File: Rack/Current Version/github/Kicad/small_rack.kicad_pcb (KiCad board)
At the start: 4 copper layers, 188 parts, among them J1 MOLEX_0015244745, J1001 HOLE_BP, J1002 HOLE_BP, J1003 HOLE_BP, J1004 HOLE_BP, J1005 HOLE_BP, J1006 HOLE_BP, J1007 HOLE_BP, J1008 HOLE_BP, J1009 HOLE_BP, J1010 HOLE_BP, J1011 HOLE_BP, J1012 HOLE_BP, J1013 HOLE_BP, J1014 HOLE_BP, J1015 HOLE_BP, J1016 HOLE_BP, J1017 HOLE_BP, J1018 HOLE_BP, J1019 HOLE_BP, J1020 HOLE_BP, J1021 SLIDER, J1022 SLIDER, J2 USB_CONNEC, K1 CONN_3, P1 CONN_8, U1 USB_CONNEC, U10 SN65LVDM176DGK, U11 TPS2044BDR, U12 CY7C65631-56LTXC, U13 USBLC6-2, U14 USBLC6-2, U15 USBLC6-2, U16 USBLC6-2, U17 USBLC6-2, U18 TPS2044BDR, U19 CY7C65631-56LTXC, U2 TE-8-1393640-3, U20 USBLC6-2, U21 USBLC6-2, U22 USBLC6-2, U23 USBLC6-2, U24 USBLC6-2, U25 CUBIEBOARD, U26 NCP1117, U27 LM73-0, U28 ATMEGA32U4, U29 ACS713, U3 TE-8-1393640-3, U4 R-535.0PA, U5 MAX1685, U6 TE-8-1393640-3, U7 TE-8-1393640-3, U8 TE-8-1393640-3, U9 FOX924B, X1 24MHz, X2 24MHz, X3 16MHz

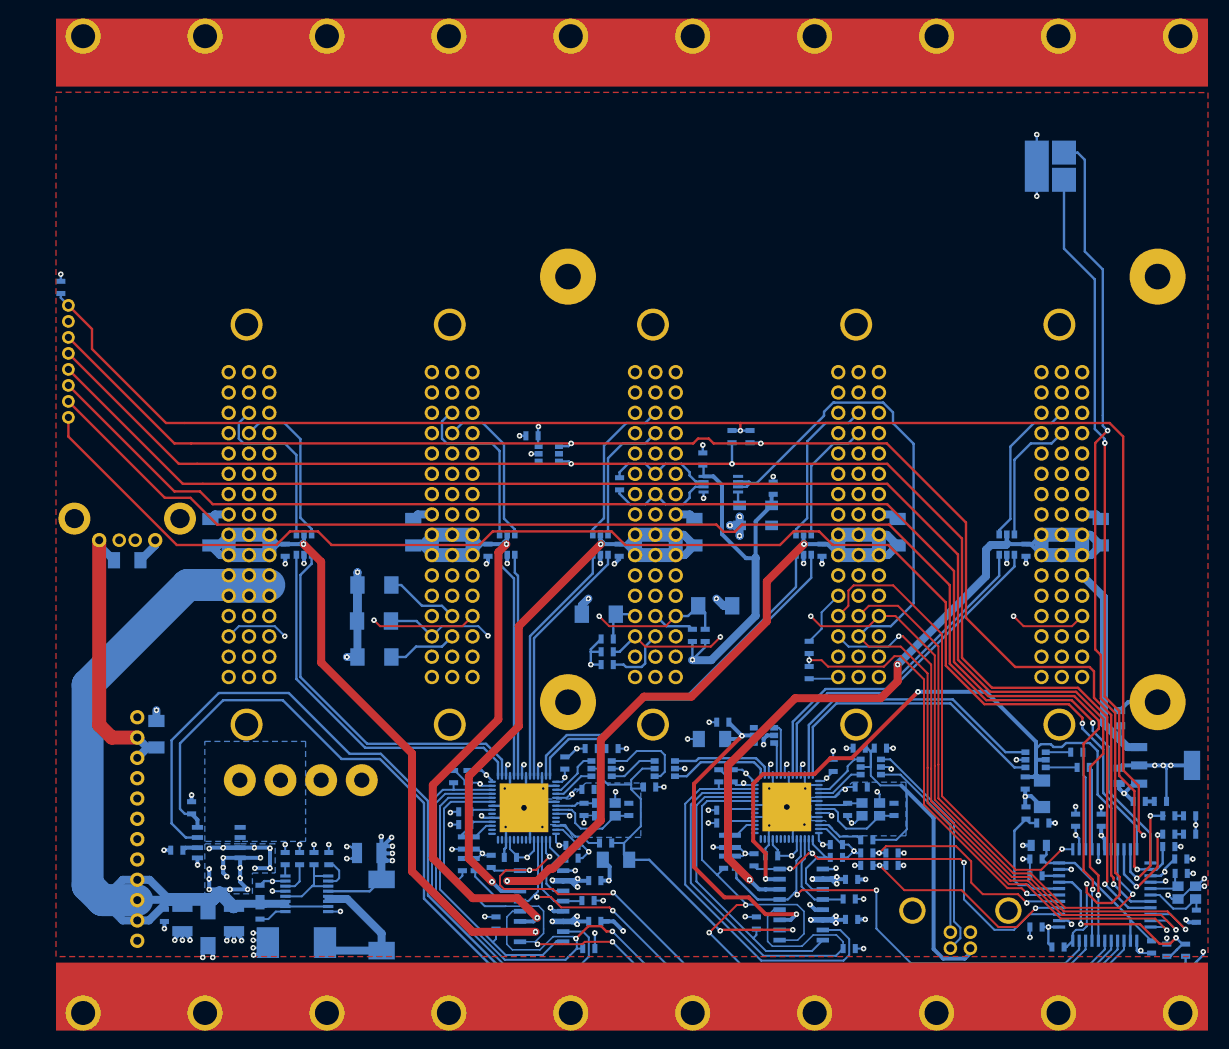
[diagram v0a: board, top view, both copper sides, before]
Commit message: current rack files
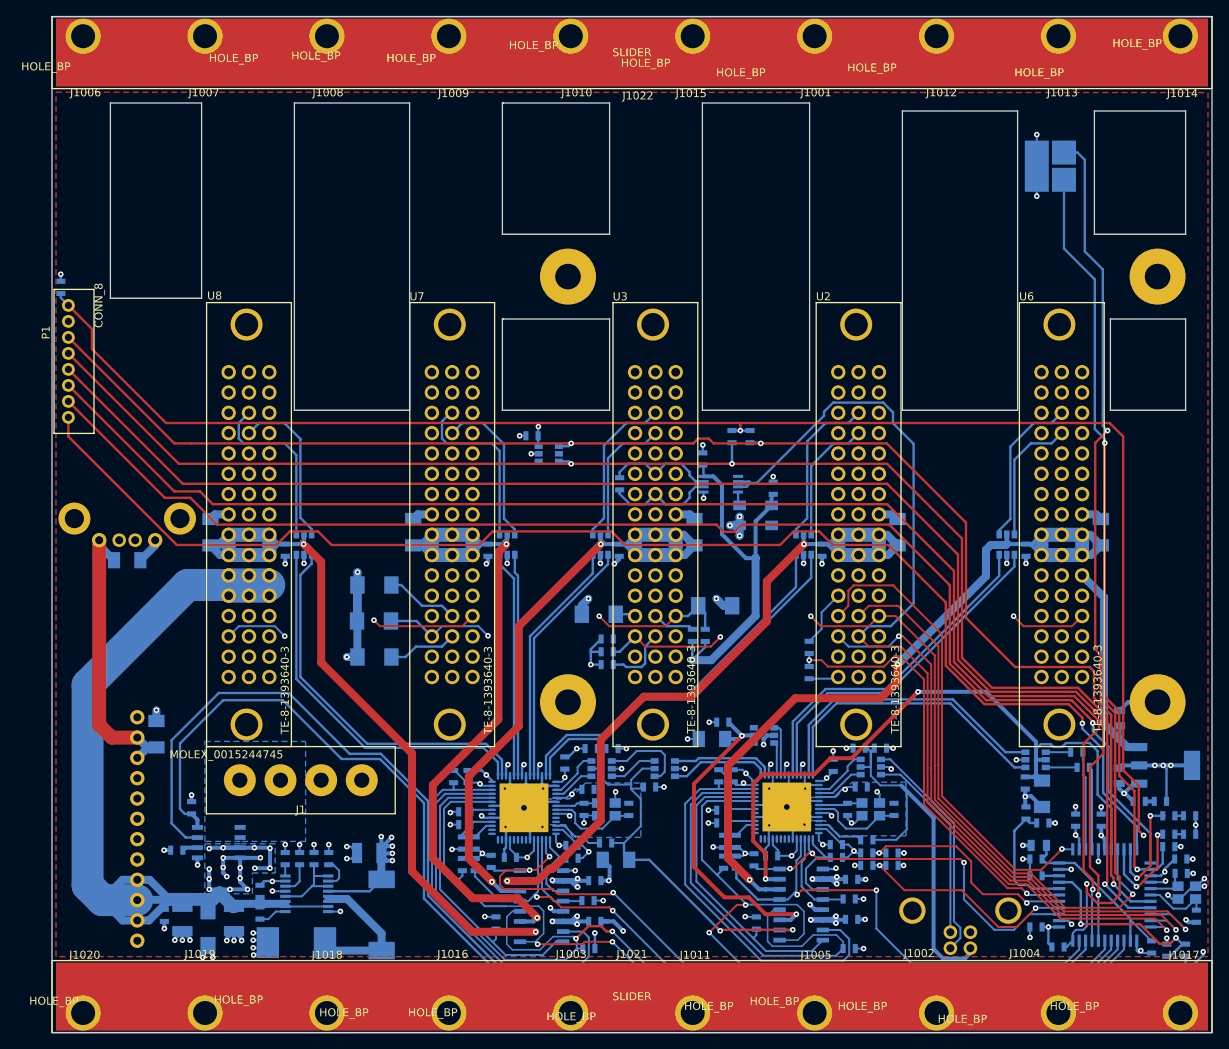
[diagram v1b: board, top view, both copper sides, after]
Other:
- board outline added: 145 x 127 mm
